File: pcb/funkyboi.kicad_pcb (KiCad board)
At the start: 4 copper layers, 78.1 x 56.2 mm, 70 parts, among them J1 Conn_01x10, J10 Conn_01x01, J11 Conn_01x01, J12 Conn_01x02, J13 Conn_01x02, J14 Conn_01x02, J15 Conn_01x01, J16 Conn_01x01, J17 Conn_01x01, J18 Conn_01x02, J19 Conn_01x01, J20 Conn_01x01, J3 Conn_01x05, J4 Conn_01x10, J5 Conn_Pi_SWD, J6 Conn_Pi_UART, J7 LCD_ST7789, J8 I2S_AUDIO, J9 Conn_01x02, Q1 BSS84, SW1 SW_RESET, SW10 START, SW2 SW_BOOTSEL, SW3 UP, SW4 LEFT, SW5 RIGHT, SW6 DOWN, SW7 B, SW8 A, SW9 SELECT, U1 W25Q128JVPIQ, U2 ME4055, U3 ME6211, U4 FLASH or PSRAM, U5 RP235x-B, Y1 CM4012M00012001

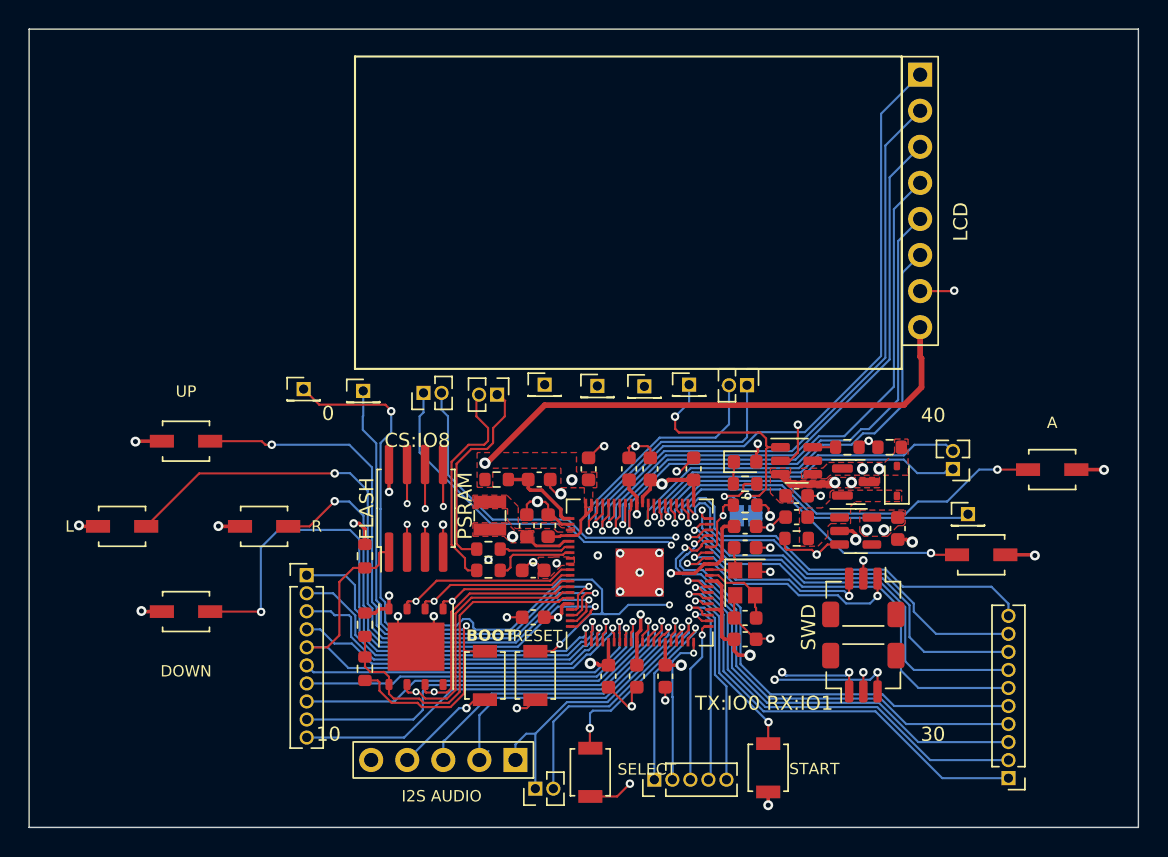
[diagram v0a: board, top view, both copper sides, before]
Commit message: revision 1 update
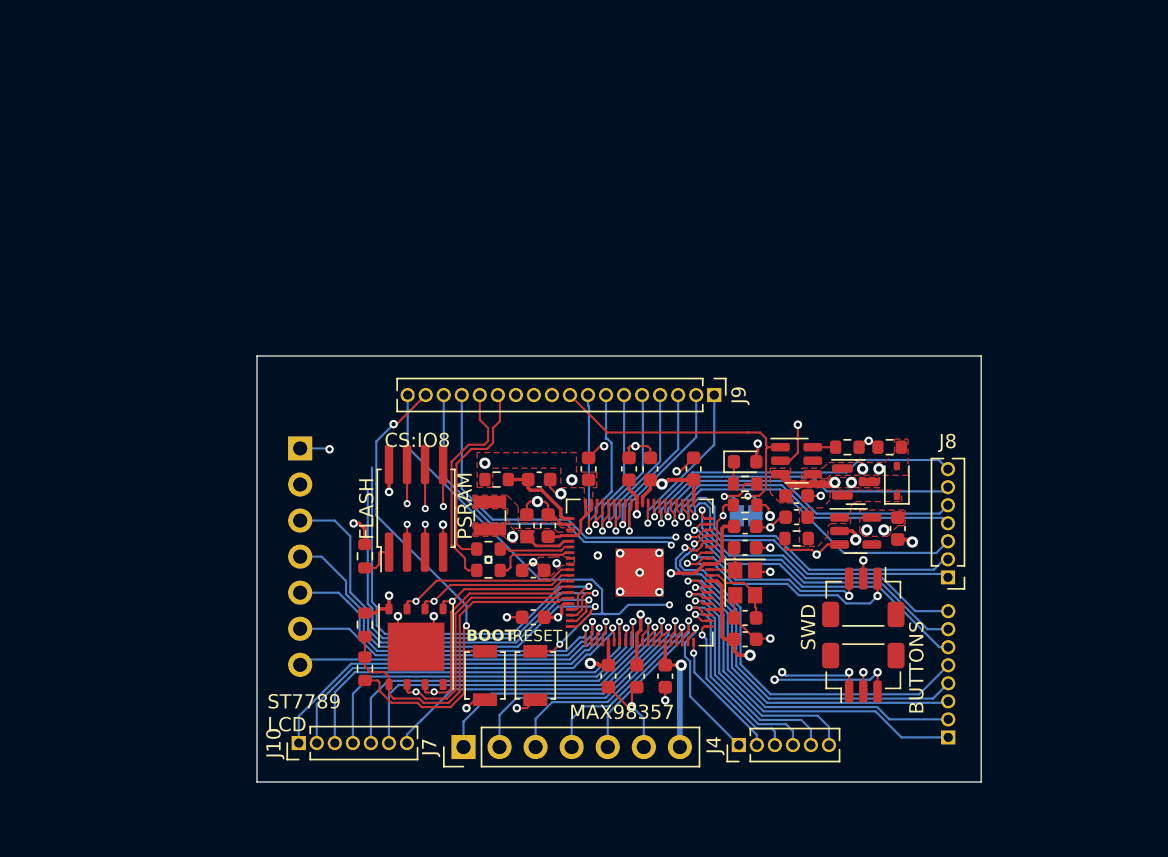
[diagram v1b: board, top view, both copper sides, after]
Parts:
- removed J11, J15, J16, J17, J19, J20: Conn_01x01, Connector_PinHeader_1.27mm:PinHeader_1x01_P1.27mm_Vertical
- removed J12, J13, J14, J18: Conn_01x02, Connector_PinHeader_1.27mm:PinHeader_1x02_P1.27mm_Vertical
- removed J3: Conn_01x05, Connector_PinHeader_1.27mm:PinHeader_1x05_P1.27mm_Vertical
- removed SW10: START, Button_Switch_SMD:SW_SPST_B3U-1000P
- removed SW3: UP, Button_Switch_SMD:SW_SPST_B3U-1000P
- removed SW4: LEFT, Button_Switch_SMD:SW_SPST_B3U-1000P
- removed SW5: RIGHT, Button_Switch_SMD:SW_SPST_B3U-1000P
- removed SW6: DOWN, Button_Switch_SMD:SW_SPST_B3U-1000P
- removed SW7: B, Button_Switch_SMD:SW_SPST_B3U-1000P
- removed SW8: A, Button_Switch_SMD:SW_SPST_B3U-1000P
- removed SW9: SELECT, Button_Switch_SMD:SW_SPST_B3U-1000P
- added J2: ST7789, Connector_PinSocket_2.54mm:PinSocket_1x07_P2.54mm_Vertical, B.Cu at (149.0, 108.5)
- J1: value Conn_01x10 -> BUTTONS; footprint Connector_PinHeader_1.27mm:PinHeader_1x10_P1.27mm_Vertical -> Connector_PinHeader_1.27mm:PinHeader_1x08_P1.27mm_Vertical; moved to B.Cu
- J10: value Conn_01x01 -> Conn_01x07; footprint Connector_PinHeader_1.27mm:PinHeader_1x01_P1.27mm_Vertical -> Connector_PinHeader_1.27mm:PinHeader_1x07_P1.27mm_Vertical
- J4: value Conn_01x10 -> Conn_01x06; footprint Connector_PinHeader_1.27mm:PinHeader_1x10_P1.27mm_Vertical -> Connector_PinHeader_1.27mm:PinHeader_1x06_P1.27mm_Vertical
- J7: value LCD_ST7789 -> MAX98357; footprint Connector_PinHeader_2.54mm:PinHeader_1x08_P2.54mm_Vertical -> Connector_PinHeader_2.54mm:PinHeader_1x07_P2.54mm_Vertical
- J8: value I2S_AUDIO -> Conn_01x07; footprint Connector_PinHeader_2.54mm:PinHeader_1x05_P2.54mm_Vertical -> Connector_PinHeader_1.27mm:PinHeader_1x07_P1.27mm_Vertical
- J9: value Conn_01x02 -> Conn_01x18; footprint Connector_PinHeader_1.27mm:PinHeader_1x02_P1.27mm_Vertical -> Connector_PinHeader_1.27mm:PinHeader_1x18_P1.27mm_Vertical
- U5: value RP235x-B -> RP2350B
- moved J7 57.2 mm to (160.5, 129.5), turned to 90 degrees
- moved J10 49.8 mm to (148.9, 129.3), turned to 90 degrees
- moved J1 46.6 mm to (194.7, 128.9)
- moved J8 33.1 mm to (194.7, 117.6)
- moved J4 19.1 mm to (179.9, 129.4), turned to 90 degrees
- moved J9 17.6 mm to (178.2, 104.8), turned to -90 degrees
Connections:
- J1 pad 1: /GPIO4 -> /GPIO25
- J1 pad 2: /GPIO5 -> /GPIO26
- J1 pad 3: /GPIO6 -> /GPIO27
- J1 pad 4: /GPIO7 -> /GPIO28
- J1 pad 5: /GPIO8 -> /GPIO29
- J1 pad 6: /GPIO9 -> /GPIO30
- J1 pad 7: /GPIO10 -> /GPIO31
- J1 pad 8: /GPIO11 -> /GPIO32
- J10 pad 1: /GPIO36 -> /GPIO7
- J4 pad 1: /GPIO25 -> /GPIO19
- J4 pad 2: /GPIO26 -> /GPIO20
- J4 pad 3: /GPIO27 -> /GPIO21
- J4 pad 4: /GPIO28 -> /GPIO22
- J4 pad 5: /GPIO29 -> /GPIO23
- J4 pad 6: /GPIO30 -> /GPIO24
- J7 pad 1: /GPIO45 -> /GPIO14
- J7 pad 2: /GPIO44 -> /BCLK
- J7 pad 3: /GPIO43 -> /DIN
- J7 pad 4: /GPIO42 -> /GAIN
- J7 pad 5: /GPIO41 -> /GPIO18
- J7 pad 6: /GPIO40 -> GND
- J7 pad 7: GND -> +3V3
- J8 pad 1: /GPIO16 -> /GPIO33
- J8 pad 2: /GPIO15 -> /GPIO34
- J8 pad 3: /GPIO14 -> /GPIO35
- J8 pad 4: GND -> /GPIO36
- J8 pad 5: +3V3 -> /GPIO37
- J9 pad 1: /GPIO38 -> /GPIO40
- J9 pad 2: /GPIO39 -> /GPIO41
- U5 pad 14: /GPIO15 -> /BCLK
- U5 pad 16: /GPIO16 -> /DIN
- U5 pad 17: /GPIO17 -> /GAIN
- U5 pad 2: /GPIO5 -> /DC
- U5 pad 3: /GPIO6 -> /BLK
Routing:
- net +3V3: track 177.8 -> 134.2 mm
- net /GPIO45: track 48.8 -> 12.4 mm
- net /GPIO44: track 45.1 -> 12.0 mm
- net /GPIO43: track 43.3 -> 13.0 mm
- net /GPIO42: track 40.6 -> 12.3 mm
- net /GPIO5: track 25.8 -> 0.00 mm, vias 1 -> 0
- net /GPIO41: track 39.3 -> 13.6 mm
- net /GPIO6: track 25.1 -> 0.00 mm, vias 1 -> 0
- net /DC: track 0.00 -> 24.4 mm, vias 0 -> 1
- net /BLK: track 0.00 -> 23.4 mm, vias 0 -> 1
- net /GPIO16: track 23.1 -> 0.00 mm, vias 1 -> 0
- net /GPIO40: track 34.4 -> 12.4 mm
- net /GPIO15: track 21.7 -> 0.00 mm, vias 1 -> 0
- net /~{RESET}: track 66.3 -> 47.9 mm, vias 4 -> 3
- net /BCLK: track 0.00 -> 18.4 mm, vias 0 -> 1
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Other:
- board size 78.1 x 56.2 mm -> 51 x 30 mm
- board text added: "+3V3"
- board text added: "13"
- board text added: "14/LRC"
- board text added: "15/BCLK"
- board text added: "16/DIN"
- board text added: "17/GAIN"
- board text added: "18/SD"
- board text added: "19"
- board text added: "24"
- board text added: "33"
- board text added: "39"
- board text added: "7"
- board text added: "BUTTONS"
- board text added: "GND"
- board text added: "GPIO40 ADC"
- board text added: "GPIO47 ADC"
- board text added: "MAX98357"
- board text added: "ST7789"
- board text added: "ST7789 LCD"
- board text added: "ahoy!"
- board text removed: "0"
- board text removed: "10"
- board text removed: "15"
- board text removed: "20"
- board text removed: "25"
- board text removed: "30"
- board text removed: "35"
- board text removed: "40"
- board text removed: "47"
- board text removed: "5"
- board text removed: "A"
- board text removed: "DOWN"
- board text removed: "I2S AUDIO"
- board text removed: "L"
- board text removed: "LCD"
- board text removed: "R"
- board text removed: "SELECT"
- board text removed: "START"
- board text removed: "TX:IO0 RX:IO1"
- board text removed: "UP"
